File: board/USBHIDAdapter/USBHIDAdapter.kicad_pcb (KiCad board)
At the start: 4 copper layers, 22.3 x 27.9 mm, 15 parts, among them J1 DE9_Plug, J2 Conn_01x04, J3 USB_1, U1 CH32V203C8T6-CH32V103C, U2 LM1117MP-3.3, Y1 Resonator

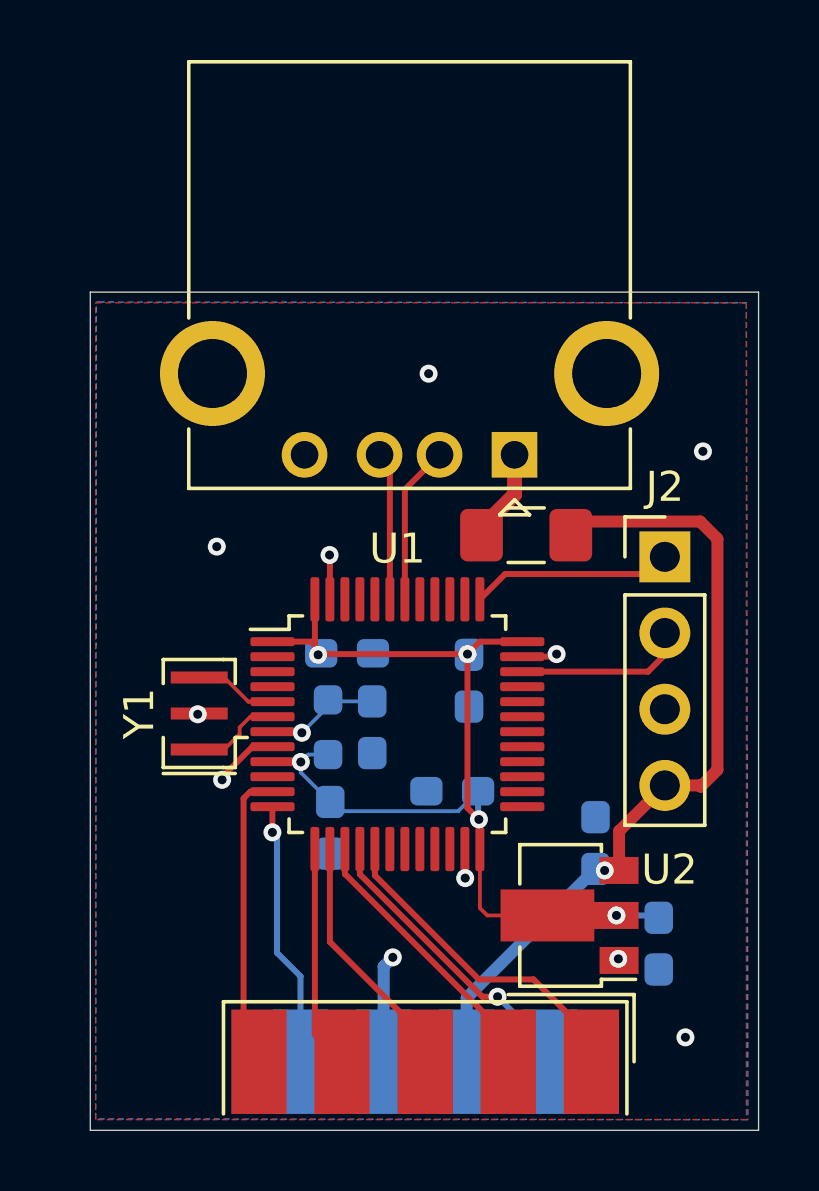
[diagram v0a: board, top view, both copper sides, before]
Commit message: Source code, board and gerbers
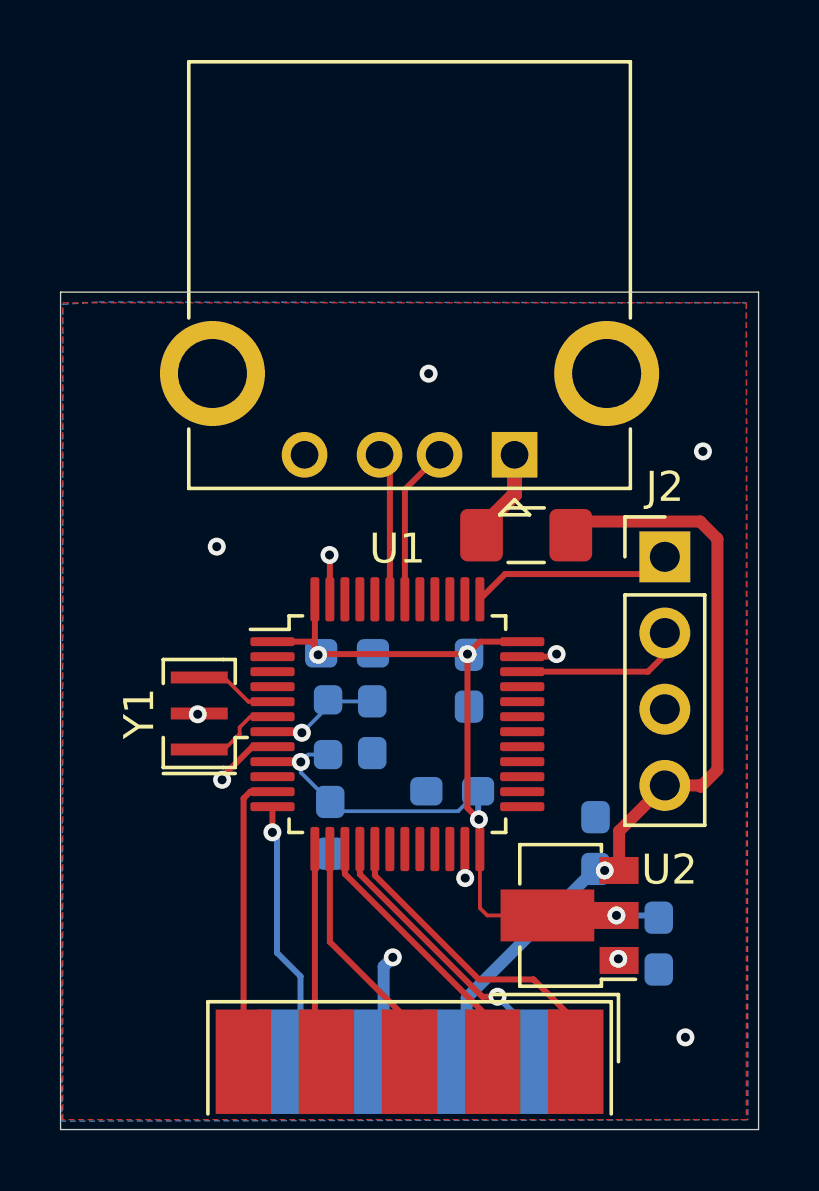
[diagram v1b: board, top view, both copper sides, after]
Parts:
- moved J1 0.52 mm to (130.2, 101.5)
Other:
- board size 22.3 x 27.9 mm -> 23.3 x 27.9 mm
- copper layers 4 -> 2
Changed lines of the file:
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@@
   (layers
     (0 "F.Cu" signal "Front")
-    (1 "In1.Cu" signal)
-    (2 "In2.Cu" signal)
     (31 "B.Cu" signal "Back")
     (34 "B.Paste" user)
@@
       (layer "F.Mask" (type "Top Solder Mask") (thickness 0.01))
       (layer "F.Cu" (type "copper") (thickness 0.035))
-      (layer "dielectric 1" (type "core") (thickness 1.51) (material "FR4") (epsilon_r 4.5) (loss_tangent 0.02))
-      (layer "In1.Cu" (type "copper") (thickness 0.035))
-      (layer "dielectric 2" (type "prepreg") (thickness 1.51) (material "FR4") (epsilon_r 4.5) (loss_tangent 0.02))
-      (layer "In2.Cu" (type "copper") (thickness 0.035))
-      (layer "dielectric 3" (type "core") (thickness 1.51) (material "FR4") (epsilon_r 4.5) (loss_tangent 0.02))
+      (layer "dielectric 1" (type "core") (thickness 4.6) (material "FR4") (epsilon_r 4.5) (loss_tangent 0.02))
       (layer "B.Cu" (type "copper") (thickness 0.035))
       (layer "B.Mask" (type "Bottom Solder Mask") (thickness 0.01))
@@
       (outputformat 1)
       (mirror false)
-      (drillshape 1)
+      (drillshape 0)
       (scaleselection 1)
-      (outputdirectory "")
+      (outputdirectory "../gerbers")
     )
   )
@@
     (fp_line (start 1.6 0.8) (end -1.6 0.8)
       (stroke (width 0.1) (type solid)) (layer "F.Fab"))
-    (pad "1" smd roundrect (at -1.4875 0) (size 1.425 1.75) (layers "F.Cu" "F.Paste" "F.Mask") (roundrect_rratio 0.175439)
+    (pad "1" smd roundrect (at -1.4875 0) (size 1.425 1.75) (layers "F.Cu" "F.Paste" "F.Mask") (roundrect_rratio 0.1754392982)
       (net 5 "Net-(J3-VBUS)") (pintype "passive"))
-    (pad "2" smd roundrect (at 1.4875 0) (size 1.425 1.75) (layers "F.Cu" "F.Paste" "F.Mask") (roundrect_rratio 0.175439)
+    (pad "2" smd roundrect (at 1.4875 0) (size 1.425 1.75) (layers "F.Cu" "F.Paste" "F.Mask") (roundrect_rratio 0.1754392982)
       (net 3 "+5V") (pintype "passive"))
     (model "${KICAD6_3DMODEL_DIR}/Fuse.3dshapes/Fuse_1206_3216Metric.wrl"
@@
   )
   (footprint "Connector_Dsub:DSUB-9_Female_EdgeMount_P2.77mm" (layer "F.Cu")
-    (at 130.695 101.4984)
+    (at 130.175 101.4984)
     (descr "9-pin D-Sub connector, solder-cups edge-mounted, female, x-pin-pitch 2.77mm, distance of mounting holes 25mm, see https://disti-assets.s3.amazonaws.com/tonar/files/datasheets/16730.pdf")
     (tags "9-pin D-Sub connector edge mount solder cup female x-pin-pitch 2.77mm mounting holes distance 25mm")
@@
     )
   )
-  (gr_rect (start 119.5324 75.8444) (end 141.8082 103.7844)
+  (gr_rect (start 118.5418 75.8444) (end 141.8082 103.759)
     (stroke (width 0.0381) (type default)) (fill none) (layer "Edge.Cuts"))
   (segment (start 132.5186 87.4962) (end 132.1054 87.9094) (width 0.2) (layer "F.Cu") (net 1))
@@
     (polygon
       (pts
-        (xy 119.7102 76.2)
+        (xy 118.618 76.2)
         (xy 141.4018 76.2)
         (xy 141.4018 103.4288)
-        (xy 119.7102 103.4288)
+        (xy 118.618 103.4288)
       )
     )
@@
         (xy 141.4018 76.2)
         (xy 141.4526 103.4288)
-        (xy 119.7102 103.4034)
-        (xy 119.7356 76.1746)
+        (xy 118.5926 103.4796)
+        (xy 118.618 76.2508)
       )
     )
